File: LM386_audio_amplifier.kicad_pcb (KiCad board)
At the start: 2 copper layers, 65.5 x 45.7 mm, 16 parts, among them J1 Conn_01x02_Female, Q1 2N3904, U1 LM386

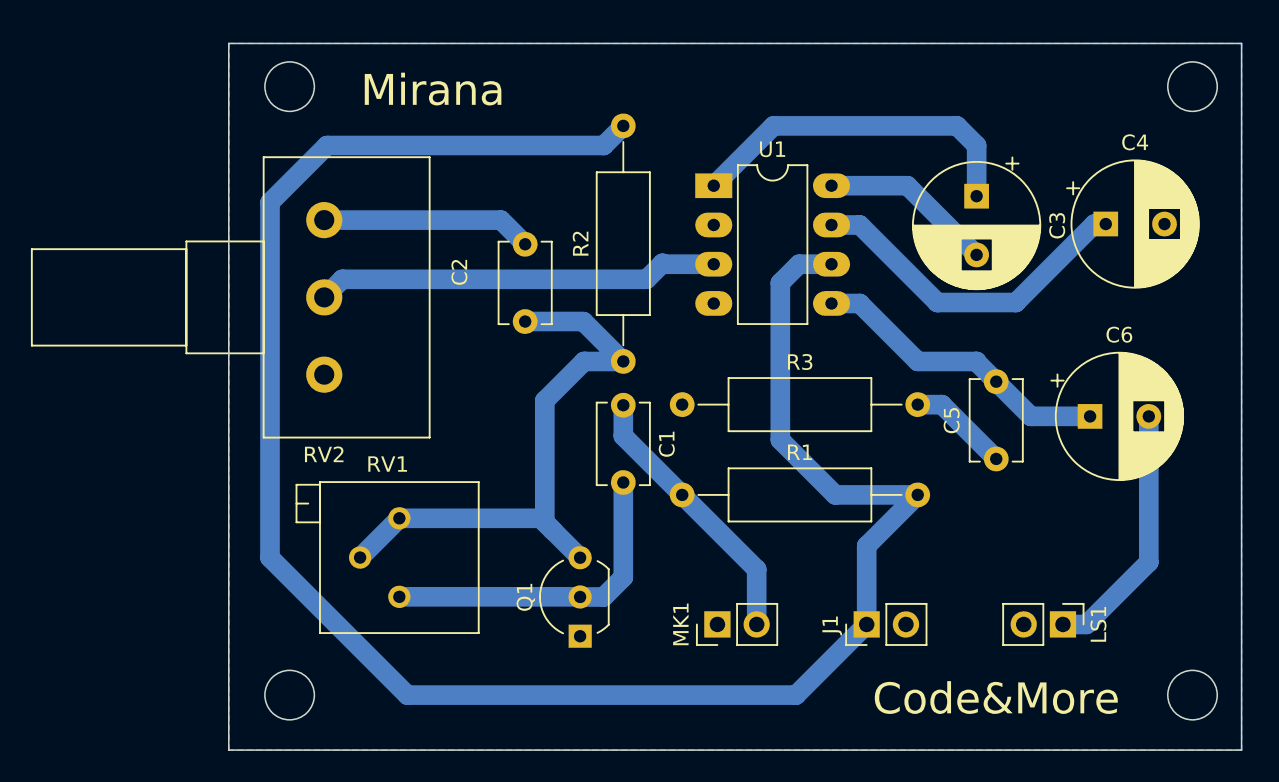
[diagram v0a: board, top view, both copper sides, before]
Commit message: some improvements
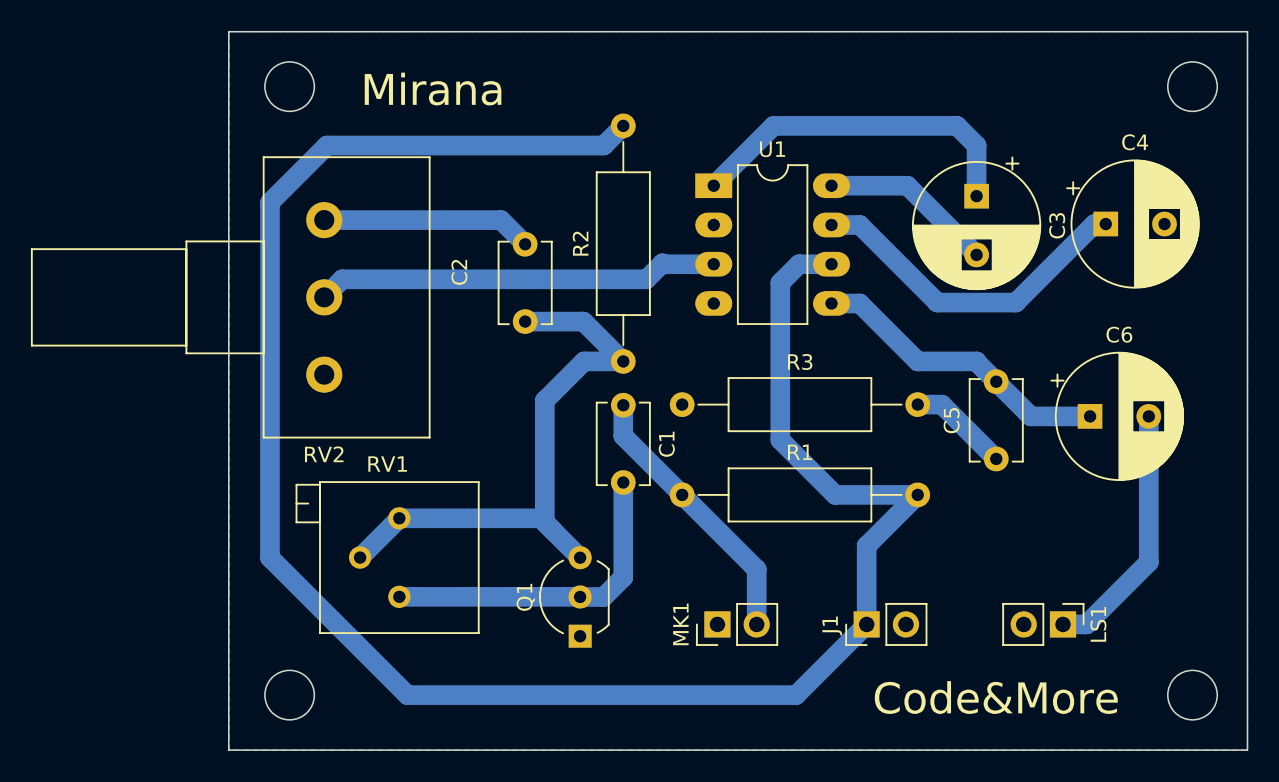
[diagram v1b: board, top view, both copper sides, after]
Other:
- board size 65.5 x 45.7 mm -> 65.9 x 46.5 mm
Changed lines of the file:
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@@
     (pad_to_mask_clearance 0)
     (pcbplotparams
-      (layerselection 0x00010fc_ffffffff)
+      (layerselection 0x0000020_7ffffffe)
       (disableapertmacros false)
       (usegerberextensions false)
@@
       (sketchpadsonfab false)
       (subtractmaskfromsilk false)
-      (outputformat 1)
-      (mirror false)
-      (drillshape 1)
+      (outputformat 4)
+      (mirror true)
+      (drillshape 2)
       (scaleselection 1)
-      (outputdirectory "")
+      (outputdirectory "C:/Users/Mirana/Desktop/lm386/")
     )
   )
@@
   )
   (gr_circle (center 149.86 39.37) (end 151.46 39.37) (layer "Edge.Cuts") (width 0.1) (fill none))
-  (gr_rect (start 87.503 36.576) (end 153.035 82.296) (layer "Edge.Cuts") (width 0.1) (fill none))
+  (gr_rect (start 87.503 35.814) (end 153.416 82.296) (layer "Edge.Cuts") (width 0.1) (fill none))
   (gr_circle (center 91.44 78.74) (end 93.04 78.74) (layer "Edge.Cuts") (width 0.1) (fill none))
   (gr_circle (center 91.44 39.37) (end 93.04 39.37) (layer "Edge.Cuts") (width 0.1) (fill none))
@@
     (polygon
       (pts
-        (xy 153.035 82.296)
+        (xy 153.416 82.296)
         (xy 87.503 82.296)
-        (xy 87.503 36.576)
-        (xy 153.035 36.576)
+        (xy 87.503 35.814)
+        (xy 153.416 35.814)
       )
     )
